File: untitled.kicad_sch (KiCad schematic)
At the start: 21 parts, among them J5 Screw_Terminal_01x02, J7 Screw_Terminal_01x02, U12 LP55231SQE_NOPB

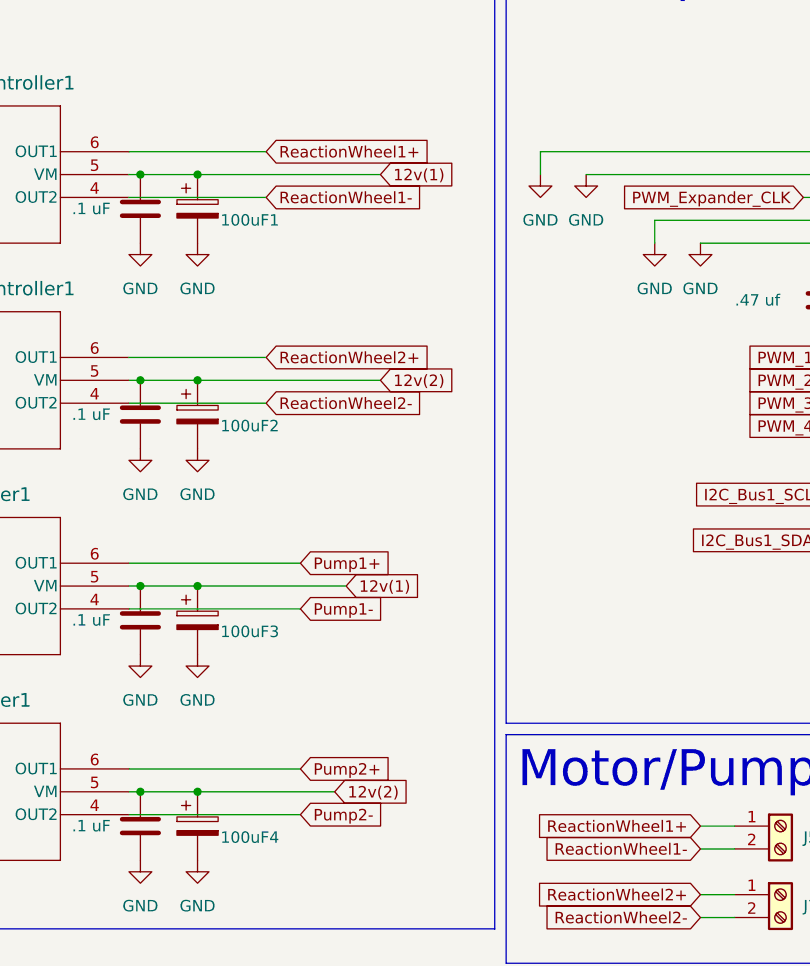
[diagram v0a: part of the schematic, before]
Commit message: Routing begin
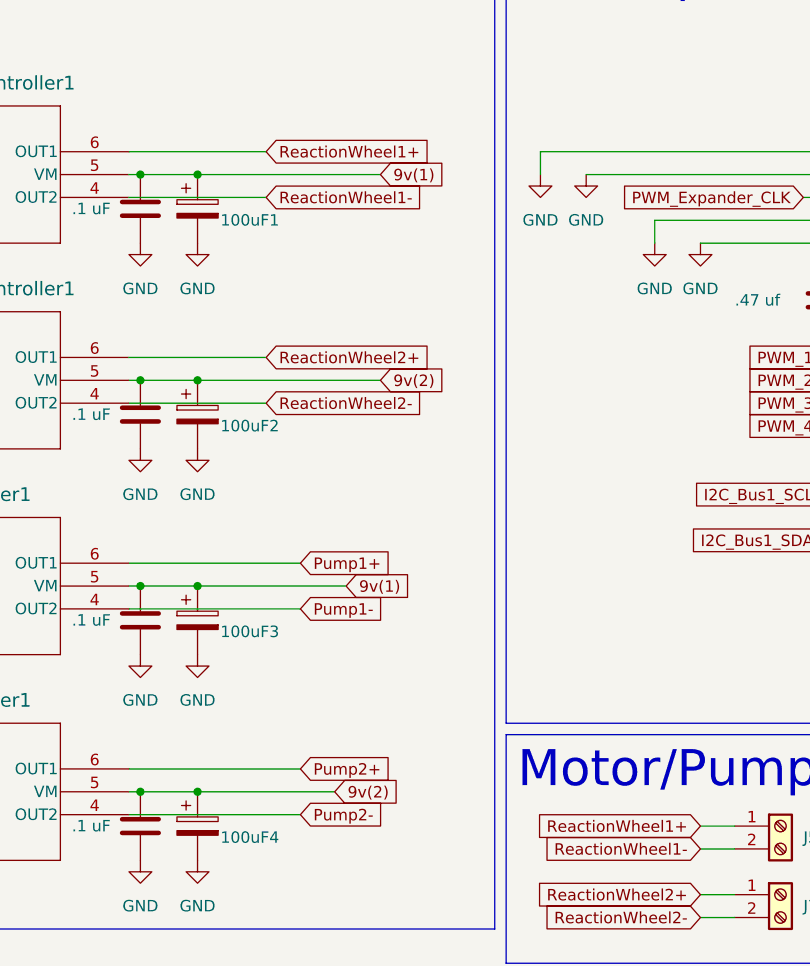
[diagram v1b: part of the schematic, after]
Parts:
- Pump1Controller1, Pump2Controller1, ReactionWheel1Controller1, ReactionWheel2Controller1: footprint Motor_Controller:SOT6_DRV8212_TEX -> DRV8212:SOT6_DRV8212_TEX-L
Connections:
- net 12v(1) renamed 9v(1)
- net 12v(2) renamed 9v(2)
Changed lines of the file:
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@@
     )
   )
-  (global_label "12v(1)" (shape input) (at 101.6 90.17 0) (fields_autoplaced)
-    (effects (font (size 1.27 1.27)) (justify left))
-    (property "Intersheetrefs" "${INTERSHEET_REFS}" (at 110.7953 90.17 0)
-      (effects (font (size 1.27 1.27)) (justify left) hide)
-    )
-  )
-  (global_label "12v(2)" (shape input) (at 105.41 67.31 0) (fields_autoplaced)
-    (effects (font (size 1.27 1.27)) (justify left))
-    (property "Intersheetrefs" "${INTERSHEET_REFS}" (at 114.6053 67.31 0)
+  (global_label "9v(1)" (shape input) (at 101.6 90.17 0) (fields_autoplaced)
+    (effects (font (size 1.27 1.27)) (justify left))
+    (property "Intersheetrefs" "${INTERSHEET_REFS}" (at 109.5858 90.17 0)
+      (effects (font (size 1.27 1.27)) (justify left) hide)
+    )
+  )
+  (global_label "9v(2)" (shape input) (at 105.41 67.31 0) (fields_autoplaced)
+    (effects (font (size 1.27 1.27)) (justify left))
+    (property "Intersheetrefs" "${INTERSHEET_REFS}" (at 113.3958 67.31 0)
       (effects (font (size 1.27 1.27)) (justify left) hide)
     )
@@
     )
   )
-  (global_label "12v(1)" (shape input) (at 105.41 44.45 0) (fields_autoplaced)
-    (effects (font (size 1.27 1.27)) (justify left))
-    (property "Intersheetrefs" "${INTERSHEET_REFS}" (at 114.6053 44.45 0)
+  (global_label "9v(1)" (shape input) (at 105.41 44.45 0) (fields_autoplaced)
+    (effects (font (size 1.27 1.27)) (justify left))
+    (property "Intersheetrefs" "${INTERSHEET_REFS}" (at 113.3958 44.45 0)
       (effects (font (size 1.27 1.27)) (justify left) hide)
     )
@@
     )
   )
-  (global_label "12v(2)" (shape input) (at 100.33 113.03 0) (fields_autoplaced)
-    (effects (font (size 1.27 1.27)) (justify left))
-    (property "Intersheetrefs" "${INTERSHEET_REFS}" (at 109.5253 113.03 0)
+  (global_label "9v(2)" (shape input) (at 100.33 113.03 0) (fields_autoplaced)
+    (effects (font (size 1.27 1.27)) (justify left))
+    (property "Intersheetrefs" "${INTERSHEET_REFS}" (at 108.3158 113.03 0)
       (effects (font (size 1.27 1.27)) (justify left) hide)
     )
@@
       (effects (font (size 1.524 1.524)) hide)
     )
-    (property "Footprint" "Motor_Controller:SOT6_DRV8212_TEX" (at 36.83 87.63 0)
+    (property "Footprint" "DRV8212:SOT6_DRV8212_TEX-L" (at 36.83 87.63 0)
       (effects (font (size 1.27 1.27) italic) hide)
     )
@@
       (effects (font (size 1.524 1.524)) hide)
     )
-    (property "Footprint" "Motor_Controller:SOT6_DRV8212_TEX" (at 36.83 64.77 0)
+    (property "Footprint" "DRV8212:SOT6_DRV8212_TEX-L" (at 36.83 64.77 0)
       (effects (font (size 1.27 1.27) italic) hide)
     )
@@
       (effects (font (size 1.524 1.524)) hide)
     )
-    (property "Footprint" "Motor_Controller:SOT6_DRV8212_TEX" (at 36.83 41.91 0)
+    (property "Footprint" "DRV8212:SOT6_DRV8212_TEX-L" (at 36.83 41.91 0)
       (effects (font (size 1.27 1.27) italic) hide)
     )
@@
       (effects (font (size 1.524 1.524)) hide)
     )
-    (property "Footprint" "Motor_Controller:SOT6_DRV8212_TEX" (at 36.83 110.49 0)
+    (property "Footprint" "DRV8212:SOT6_DRV8212_TEX-L" (at 36.83 110.49 0)
       (effects (font (size 1.27 1.27) italic) hide)
     )

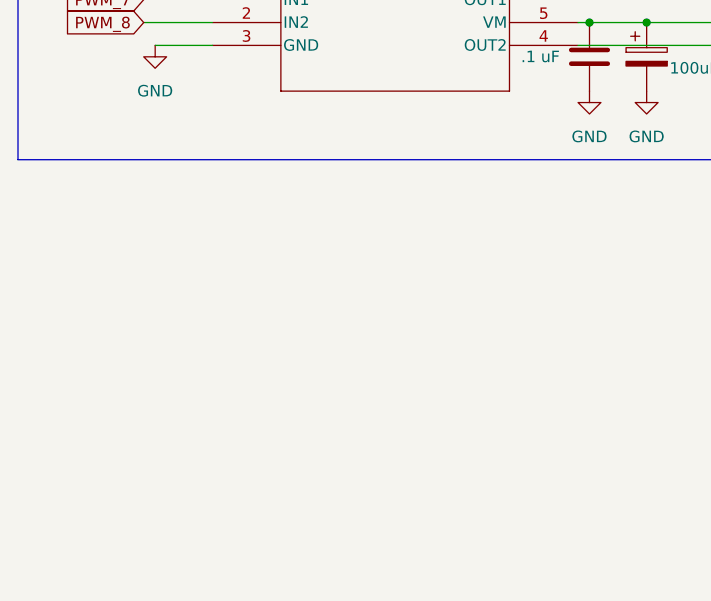
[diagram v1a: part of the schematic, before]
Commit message: Tedi Check dis over pls.
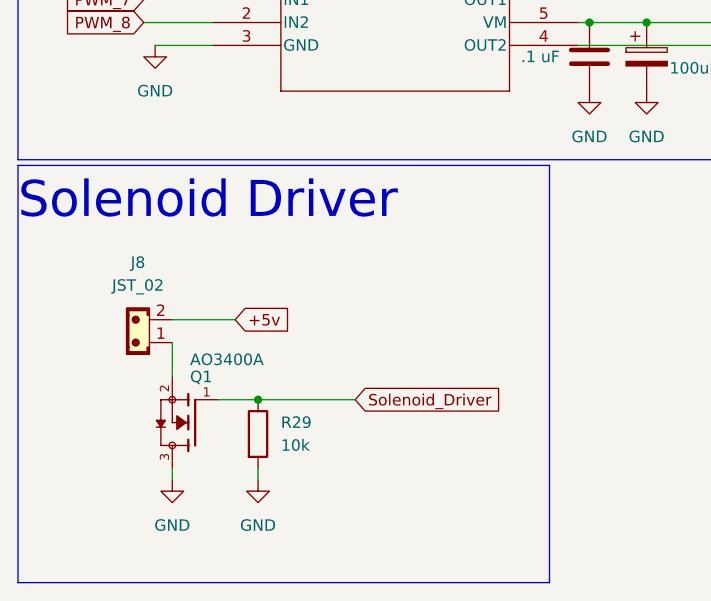
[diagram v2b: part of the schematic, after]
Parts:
- added J8: JST_02, Connector_JST:JST_EH_B2B-EH-A_1x02_P2.50mm_Vertical, symbol PCM_SL_Connectors:JST_02
- added Q1: AO3400A, N-Channel:SOT95P280X125-3N, symbol N-Channel-FET:AO3400A
- added R29: 10k, Resistor_SMD:R_0603_1608Metric_Pad0.98x0.95mm_HandSolder, symbol Device:R
- U12: footprint PWM Expander:QFN50P400X400X80-25N -> PWM_EXPANDER:RTW24_TEX
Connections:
- net +5v: now also J8.2
- net GND: now also Q1.3, R29.2
- new net: J8.1, Q1.2
- new net Solenoid_Driver: Q1.1, R29.1
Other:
- note added: "Solenoid Driver"
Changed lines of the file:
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@@
   (junction (at 78.74 44.45) (diameter 0) (color 0 0 0 0)
+  )
+  (junction (at 41.91 154.94) (diameter 0) (color 0 0 0 0)
   )
   (junction (at 85.09 90.17) (diameter 0) (color 0 0 0 0)
@@
     (stroke (width 0) (type default))
   )
+  (wire (pts (xy 39.37 146.05) (xy 32.385 146.05))
+    (stroke (width 0) (type default))
+  )
   (wire (pts (xy 30.48 92.71) (xy 36.83 92.71))
     (stroke (width 0) (type default))
@@
     (stroke (width 0) (type default))
   )
+  (wire (pts (xy 32.385 152.4) (xy 32.385 148.59))
+    (stroke (width 0) (type default))
+  )
   (wire (pts (xy 30.48 44.45) (xy 36.83 44.45))
     (stroke (width 0) (type default))
@@
     (stroke (width 0) (type default))
   )
+  (wire (pts (xy 32.385 163.83) (xy 32.385 162.56))
+    (stroke (width 0) (type default))
+  )
   (wire (pts (xy 101.6 90.17) (xy 85.09 90.17))
     (stroke (width 0) (type default))
@@
     (stroke (width 0) (type default))
   )
+  (wire (pts (xy 41.91 163.83) (xy 41.91 162.56))
+    (stroke (width 0) (type default))
+  )
   (wire (pts (xy 185.42 120.65) (xy 189.23 120.65))
     (stroke (width 0) (type default))
@@
     (stroke (width 0) (type default))
   )
+  (wire (pts (xy 37.465 154.94) (xy 41.91 154.94))
+    (stroke (width 0) (type default))
+  )
   (wire (pts (xy 78.74 90.17) (xy 77.47 90.17))
     (stroke (width 0) (type default))
@@
     (stroke (width 0) (type default))
   )
+  (wire (pts (xy 41.91 154.94) (xy 52.705 154.94))
+    (stroke (width 0) (type default))
+  )
   (wire (pts (xy 140.97 119.38) (xy 144.78 119.38))
     (stroke (width 0) (type default))
   )
   (rectangle (start 119.38 106.68) (end 205.74 132.08)
+    (stroke (width 0) (type default))
+    (fill (type none))
+  )
+  (rectangle (start 15.24 128.905) (end 74.295 175.26)
     (stroke (width 0) (type default))
     (fill (type none))
@@
     (effects (font (size 4 4)) (justify left bottom))
   )
+  (text "Solenoid Driver" (at 15.24 135.255 0)
+    (effects (font (size 4 4)) (justify left bottom))
+  )
   (global_label "Pump1-" (shape input) (at 185.42 120.65 180) (fields_autoplaced)
     (effects (font (size 1.27 1.27)) (justify right))
@@
     )
   )
+  (global_label "Solenoid_Driver" (shape input) (at 52.705 154.94 0) (fields_autoplaced)
+    (effects (font (size 1.27 1.27)) (justify left))
+    (property "Intersheetrefs" "${INTERSHEET_REFS}" (at 70.2459 154.94 0)
+      (effects (font (size 1.27 1.27)) (justify left) hide)
+    )
+  )
   (global_label "Pump2-" (shape input) (at 96.52 115.57 0) (fields_autoplaced)
     (effects (font (size 1.27 1.27)) (justify left))
@@
     (effects (font (size 1.27 1.27)) (justify left))
     (property "Intersheetrefs" "${INTERSHEET_REFS}" (at 113.3958 44.45 0)
+      (effects (font (size 1.27 1.27)) (justify left) hide)
+    )
+  )
+  (global_label "+5v" (shape input) (at 39.37 146.05 0) (fields_autoplaced)
+    (effects (font (size 1.27 1.27)) (justify left))
+    (property "Intersheetrefs" "${INTERSHEET_REFS}" (at 46.0253 146.05 0)
       (effects (font (size 1.27 1.27)) (justify left) hide)
     )
@@
     )
   )
+  (symbol (lib_id "power:GND") (at 32.385 163.83 0) (unit 1)
+    (in_bom yes) (on_board yes) (dnp no) (fields_autoplaced)
+    (property "Reference" "#PWR099" (at 32.385 170.18 0)
+      (effects (font (size 1.27 1.27)) hide)
+    )
+    (property "Value" "GND" (at 32.385 168.91 0)
+      (effects (font (size 1.27 1.27)))
+    )
+    (property "Footprint" "" (at 32.385 163.83 0)
+      (effects (font (size 1.27 1.27)) hide)
+    )
+    (property "Datasheet" "" (at 32.385 163.83 0)
+      (effects (font (size 1.27 1.27)) hide)
+    )
+    (pin "1")
+    (instances
+      (project "Watersphere mobo"
+        (path "/c4a63ad0-0af5-4f61-bde7-7fb53fc8413c/f3a59c99-c5f5-41f4-9185-d6e5a8c7c677"
+          (reference "#PWR099") (unit 1)
+        )
+      )
+    )
+  )
   (symbol (lib_id "power:GND") (at 30.48 69.85 0) (unit 1)
     (in_bom yes) (on_board yes) (dnp no) (fields_autoplaced)
@@
         (path "/c4a63ad0-0af5-4f61-bde7-7fb53fc8413c/f3a59c99-c5f5-41f4-9185-d6e5a8c7c677"
           (reference "#PWR028") (unit 1)
+        )
+      )
+    )
+  )
+  (symbol (lib_id "Device:R") (at 41.91 158.75 0) (unit 1)
+    (in_bom yes) (on_board yes) (dnp no) (fields_autoplaced)
+    (property "Reference" "R29" (at 44.45 157.48 0)
+      (effects (font (size 1.27 1.27)) (justify left))
+    )
+    (property "Value" "10k" (at 44.45 160.02 0)
+      (effects (font (size 1.27 1.27)) (justify left))
+    )
+    (property "Footprint" "Resistor_SMD:R_0603_1608Metric_Pad0.98x0.95mm_HandSolder" (at 40.132 158.75 90)
+      (effects (font (size 1.27 1.27)) hide)
+    )
+    (property "Datasheet" "~" (at 41.91 158.75 0)
+      (effects (font (size 1.27 1.27)) hide)
+    )
+    (pin "1")
+    (pin "2")
+    (instances
+      (project "Watersphere mobo"
+        (path "/c4a63ad0-0af5-4f61-bde7-7fb53fc8413c/f3a59c99-c5f5-41f4-9185-d6e5a8c7c677"
+          (reference "R29") (unit 1)
         )
       )
@@
     )
   )
+  (symbol (lib_id "PCM_SL_Connectors:JST_02") (at 28.575 147.32 180) (unit 1)
+    (in_bom yes) (on_board yes) (dnp no) (fields_autoplaced)
+    (property "Reference" "J8" (at 28.575 139.7 0)
+      (effects (font (size 1.27 1.27)))
+    )
+    (property "Value" "JST_02" (at 28.575 142.24 0)
+      (effects (font (size 1.27 1.27)))
+    )
+    (property "Footprint" "Connector_JST:JST_EH_B2B-EH-A_1x02_P2.50mm_Vertical" (at 28.575 153.67 0)
+      (effects (font (size 1.27 1.27)) hide)
+    )
+    (property "Datasheet" "" (at 28.575 153.67 0)
+      (effects (font (size 1.27 1.27)) hide)
+    )
+    (pin "1")
+    (pin "2")
+    (instances
+      (project "Watersphere mobo"
+        (path "/c4a63ad0-0af5-4f61-bde7-7fb53fc8413c/f3a59c99-c5f5-41f4-9185-d6e5a8c7c677"
+          (reference "J8") (unit 1)
+        )
+      )
+    )
+  )
   (symbol (lib_id "power:GND") (at 85.09 52.07 0) (unit 1)
     (in_bom yes) (on_board yes) (dnp no) (fields_autoplaced)
@@
     )
   )
+  (symbol (lib_id "power:GND") (at 41.91 163.83 0) (unit 1)
+    (in_bom yes) (on_board yes) (dnp no) (fields_autoplaced)
+    (property "Reference" "#PWR0100" (at 41.91 170.18 0)
+      (effects (font (size 1.27 1.27)) hide)
+    )
+    (property "Value" "GND" (at 41.91 168.91 0)
+      (effects (font (size 1.27 1.27)))
+    )
+    (property "Footprint" "" (at 41.91 163.83 0)
+      (effects (font (size 1.27 1.27)) hide)
+    )
+    (property "Datasheet" "" (at 41.91 163.83 0)
+      (effects (font (size 1.27 1.27)) hide)
+    )
+    (pin "1")
+    (instances
+      (project "Watersphere mobo"
+        (path "/c4a63ad0-0af5-4f61-bde7-7fb53fc8413c/f3a59c99-c5f5-41f4-9185-d6e5a8c7c677"
+          (reference "#PWR0100") (unit 1)
+        )
+      )
+    )
+  )
   (symbol (lib_id "PWM Expander:LP55231SQE_NOPB") (at 177.8 67.31 0) (unit 1)
     (in_bom yes) (on_board yes) (dnp no) (fields_autoplaced)
@@
       (effects (font (size 1.27 1.27)))
     )
-    (property "Footprint" "PWM Expander:QFN50P400X400X80-25N" (at 177.8 67.31 0)
+    (property "Footprint" "PWM_EXPANDER:RTW24_TEX" (at 177.8 67.31 0)
       (effects (font (size 1.27 1.27)) (justify bottom) hide)
     )
@@
         )
       )
+    )
+  )
+  (symbol (lib_id "N-Channel-FET:AO3400A") (at 34.925 157.48 180) (unit 1)
+    (in_bom yes) (on_board yes) (dnp no)
+    (property "Reference" "Q1" (at 36.83 152.4 0)
+      (effects (font (size 1.27 1.27)) (justify left))
+    )
+    (property "Value" "AO3400A" (at 42.545 150.495 0)
+      (effects (font (size 1.27 1.27)) (justify left))
+    )
+    (property "Footprint" "N-Channel:SOT95P280X125-3N" (at 34.925 157.48 0)
+      (effects (font (size 1.27 1.27)) (justify bottom) hide)
+    )
+    (property "Datasheet" "" (at 34.925 157.48 0)
+      (effects (font (size 1.27 1.27)) hide)
+    )
+    (property "MF" "Alpha &" (at 34.925 157.48 0)
+      (effects (font (size 1.27 1.27)) (justify bottom) hide)
+    )
+    (property "MAXIMUM_PACKAGE_HEIGHT" "1.25 mm" (at 34.925 157.48 0)
+      (effects (font (size 1.27 1.27)) (justify bottom) hide)
+    )
+    (property "Package" "SOT-23 Alpha &amp; Omega Semiconductor" (at 34.925 157.48 0)
+      (effects (font (size 1.27 1.27)) (justify bottom) hide)
+    )
+    (property "Price" "None" (at 34.925 157.48 0)
+      (effects (font (size 1.27 1.27)) (justify bottom) hide)
+    )
+    (property "Check_prices" "https://www.snapeda.com/parts/AO3400A/Alpha+%2526+Omega+Semiconductor+Inc./view-part/?ref=eda" (at 34.925 157.48 0)
+      (effects (font (size 1.27 1.27)) (justify bottom) hide)
+    )
+    (property "STANDARD" "IPC 7351B" (at 34.925 157.48 0)
+      (effects (font (size 1.27 1.27)) (justify bottom) hide)
+    )
+    (property "PARTREV" "L" (at 34.925 157.48 0)
+      (effects (font (size 1.27 1.27)) (justify bottom) hide)
+    )
+    (property "SnapEDA_Link" "https://www.snapeda.com/parts/AO3400A/Alpha+%2526+Omega+Semiconductor+Inc./view-part/?ref=snap" (at 34.925 157.48 0)
+      (effects (font (size 1.27 1.27)) (justify bottom) hide)
+    )
+    (property "MP" "AO3400A" (at 34.925 157.48 0)
+      (effects (font (size 1.27 1.27)) (justify bottom) hide)
+    )
+    (property "Description" "\nN-Channel 30 V 5.7A (Ta) 1.4W (Ta) Surface Mount SOT-23-3\n" (at 34.925 157.48 0)
+      (effects (font (size 1.27 1.27)) (justify bottom) hide)
+    )
+    (property "Availability" "In Stock" (at 34.925 157.48 0)
+      (effects (font (size 1.27 1.27)) (justify bottom) hide)
+    )
+    (property "MANUFACTURER" "Alpha & Omega Semiconductor" (at 34.925 157.48 0)
+      (effects (font (size 1.27 1.27)) (justify bottom) hide)
+    )
+    (pin "1")
+    (pin "2")
+    (pin "3")
+    (instances
+      (project "Watersphere mobo"
+        (path "/c4a63ad0-0af5-4f61-bde7-7fb53fc8413c/f3a59c99-c5f5-41f4-9185-d6e5a8c7c677"
+          (reference "Q1") (unit 1)
+        )
+      )
